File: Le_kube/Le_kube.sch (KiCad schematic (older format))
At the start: 1 part

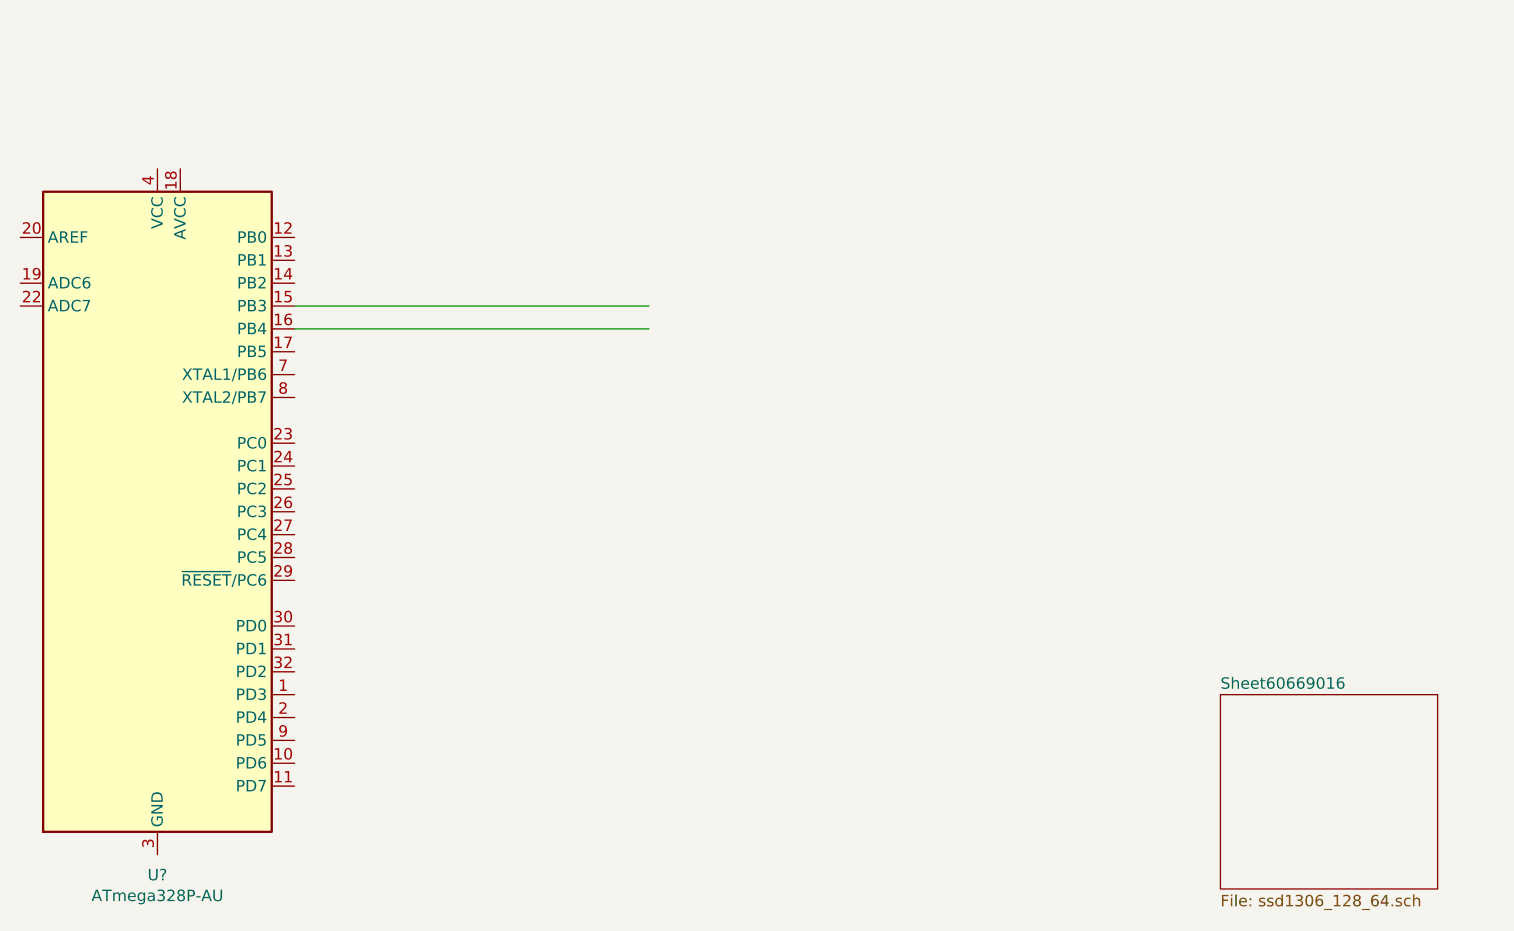
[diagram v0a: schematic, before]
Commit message: continue on kicad_ssd1306
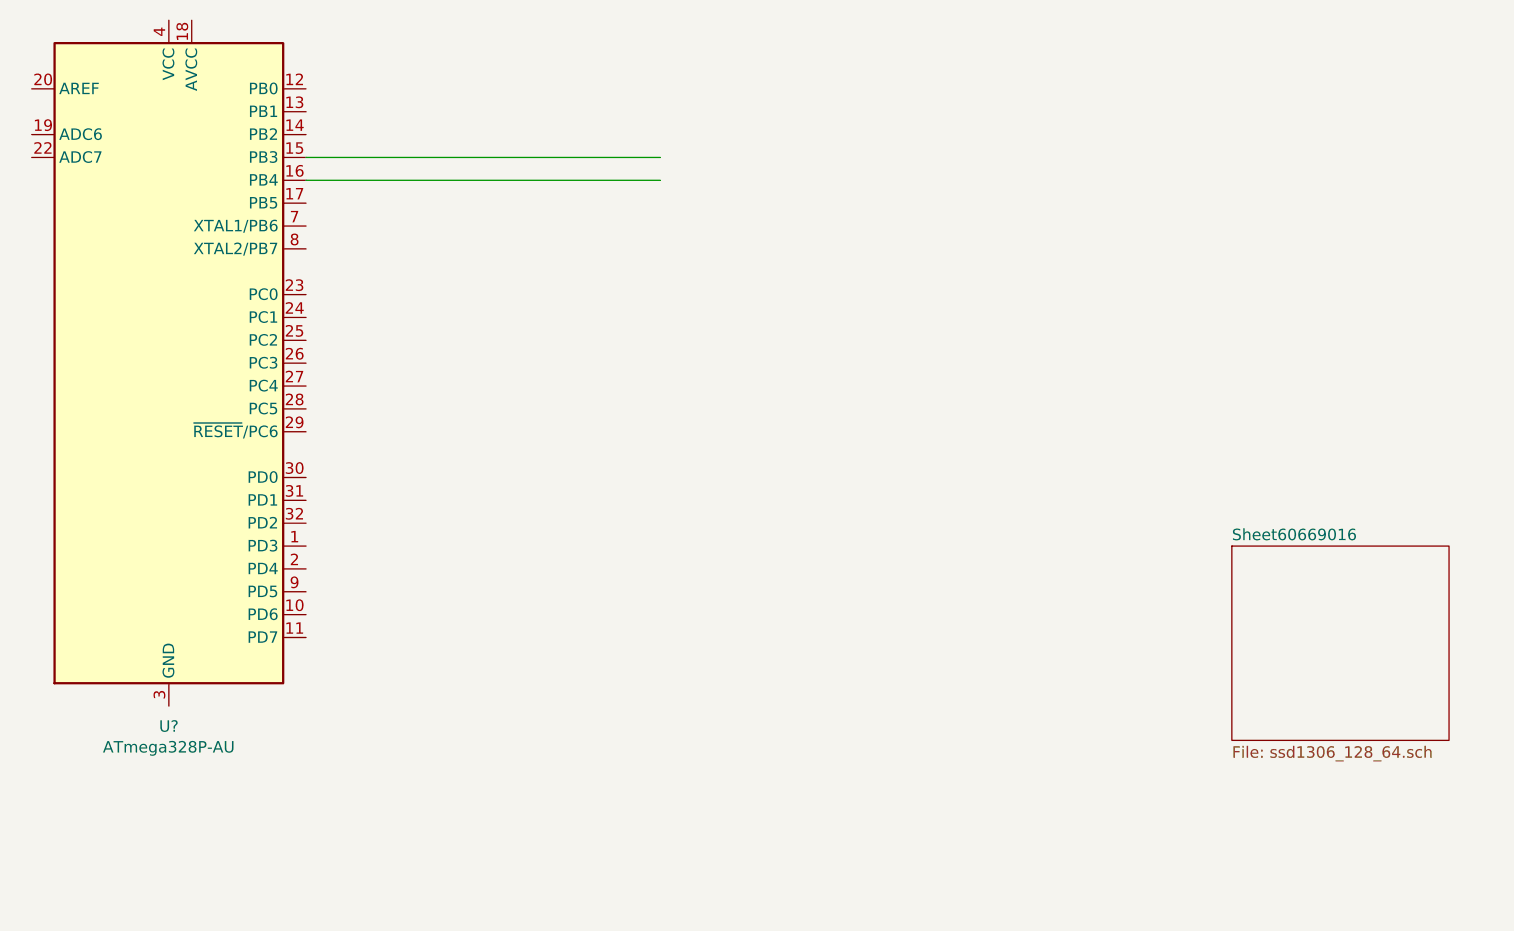
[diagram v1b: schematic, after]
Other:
- moved on the sheet: U?
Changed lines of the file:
@@
 L MCU_Microchip_ATmega:ATmega328P-AU U?
 U 1 1 606383C9
-P 2950 3400
-F 0 "U?" H 2950 1811 50  0000 C CNN
-F 1 "ATmega328P-AU" H 2950 1720 50  0000 C CNN
-F 2 "Package_QFP:TQFP-32_7x7mm_P0.8mm" H 2950 3400 50  0001 C CIN
-F 3 "http://ww1.microchip.com/downloads/en/DeviceDoc/ATmega328_P%20AVR%20MCU%20with%20picoPower%20Technology%20Data%20Sheet%2040001984A.pdf" H 2950 3400 50  0001 C CNN
-	1    2950 3400
+P 3000 2750
+F 0 "U?" H 3000 1161 50  0000 C CNN
+F 1 "ATmega328P-AU" H 3000 1070 50  0000 C CNN
+F 2 "Package_QFP:TQFP-32_7x7mm_P0.8mm" H 3000 2750 50  0001 C CIN
+F 3 "http://ww1.microchip.com/downloads/en/DeviceDoc/ATmega328_P%20AVR%20MCU%20with%20picoPower%20Technology%20Data%20Sheet%2040001984A.pdf" H 3000 2750 50  0001 C CNN
+	1    3000 2750
 	1    0    0    -1
 $EndComp
 Wire Wire Line
-	3550 2500 5100 2500
+	3600 1850 5150 1850
 Wire Wire Line
-	3550 2600 5100 2600
+	3600 1950 5150 1950
 $Sheet
-S 7600 4200 950  850
+S 7650 3550 950  850
 U 60669017
 F0 "Sheet60669016" 50
